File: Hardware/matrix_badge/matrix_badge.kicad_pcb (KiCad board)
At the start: 2 copper layers, 25.4 x 39.4 mm, 35 parts, among them J1 Conn_02x03_Odd_Even, U1 ATTINY85-20SU

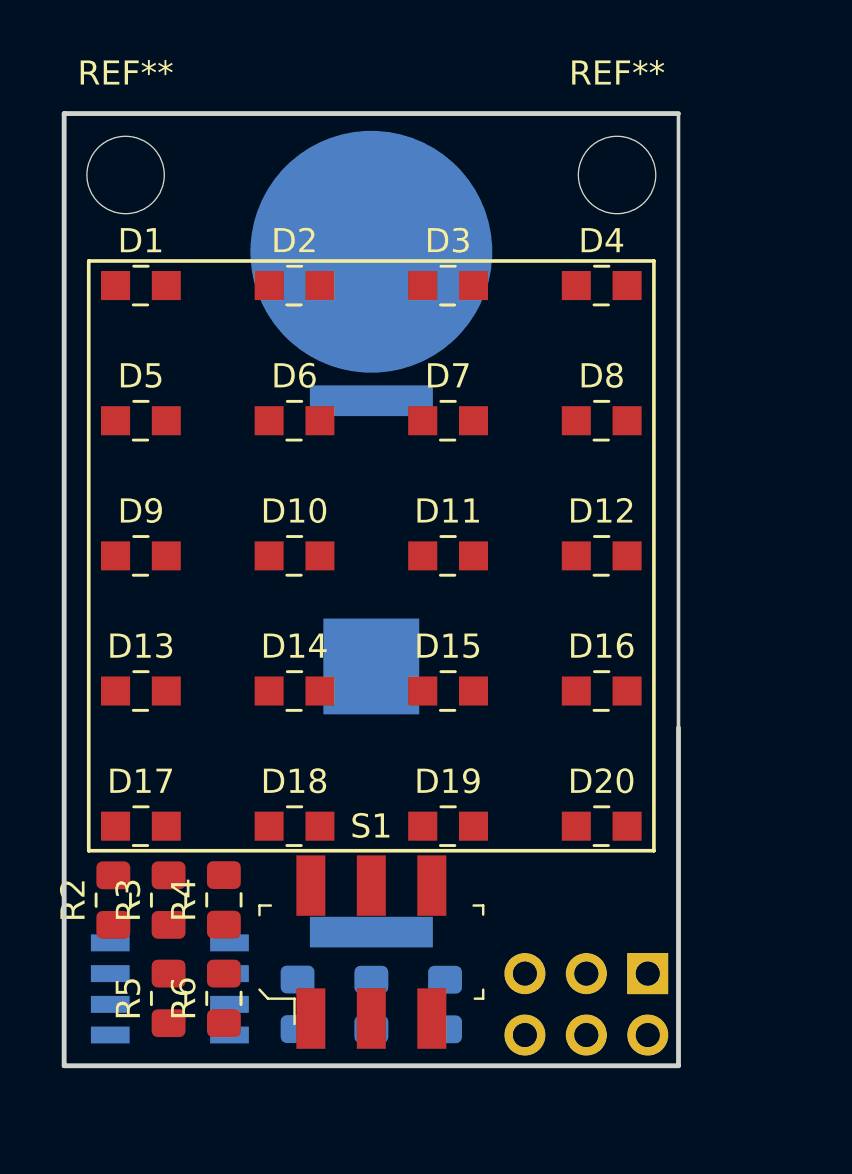
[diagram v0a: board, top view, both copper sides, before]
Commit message: Reconfigured footprint positions
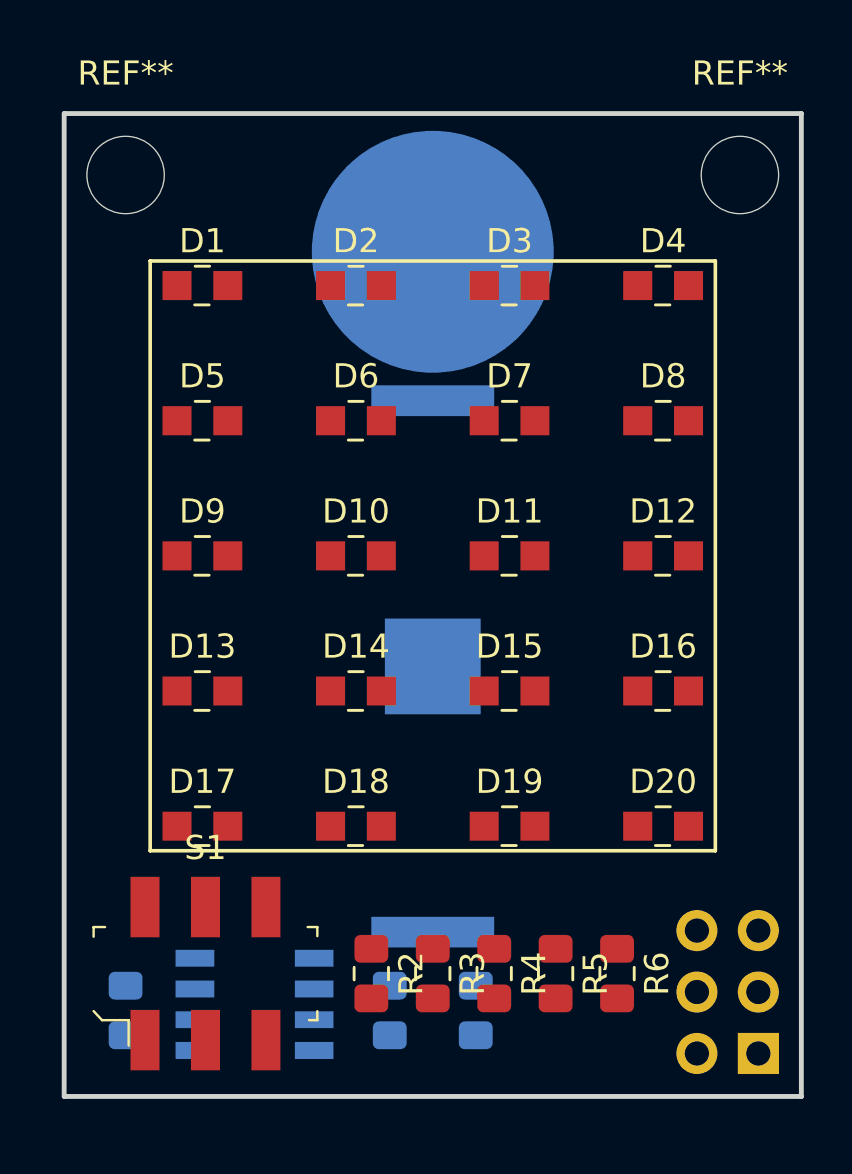
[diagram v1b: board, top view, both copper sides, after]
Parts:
- moved R6 16.3 mm to (149.9, 111.8), turned to 270 degrees
- moved R5 16.0 mm to (147.3, 111.8), turned to 270 degrees
- moved R4 11.6 mm to (144.8, 111.8), turned to 270 degrees
- moved R3 11.3 mm to (142.2, 111.8), turned to 270 degrees
- moved R2 11.1 mm to (139.7, 111.8), turned to 270 degrees
- moved C2 7.12 mm to (129.5, 113.3), turned to 270 degrees
- moved S1 6.92 mm to (132.8, 111.8)
- moved J1 5.64 mm to (155.7, 115.1), turned to 0 degrees
- moved REF** 5.08 mm to (154.9, 78.7)
- moved U1 3.56 mm to (134.9, 113.0)
- moved BT1 2.54 mm to (142.2, 99.1)
- moved REF** 2.54 mm to (142.2, 81.9)
- moved D1 2.54 mm to (132.7, 83.3)
- moved D10 2.54 mm to (139.1, 94.5)
- moved D11 2.54 mm to (145.4, 94.5)
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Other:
- board size 25.4 x 39.4 mm -> 30.5 x 40.6 mm

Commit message: Layout ALMOST done. Missing 1 gnd connection.
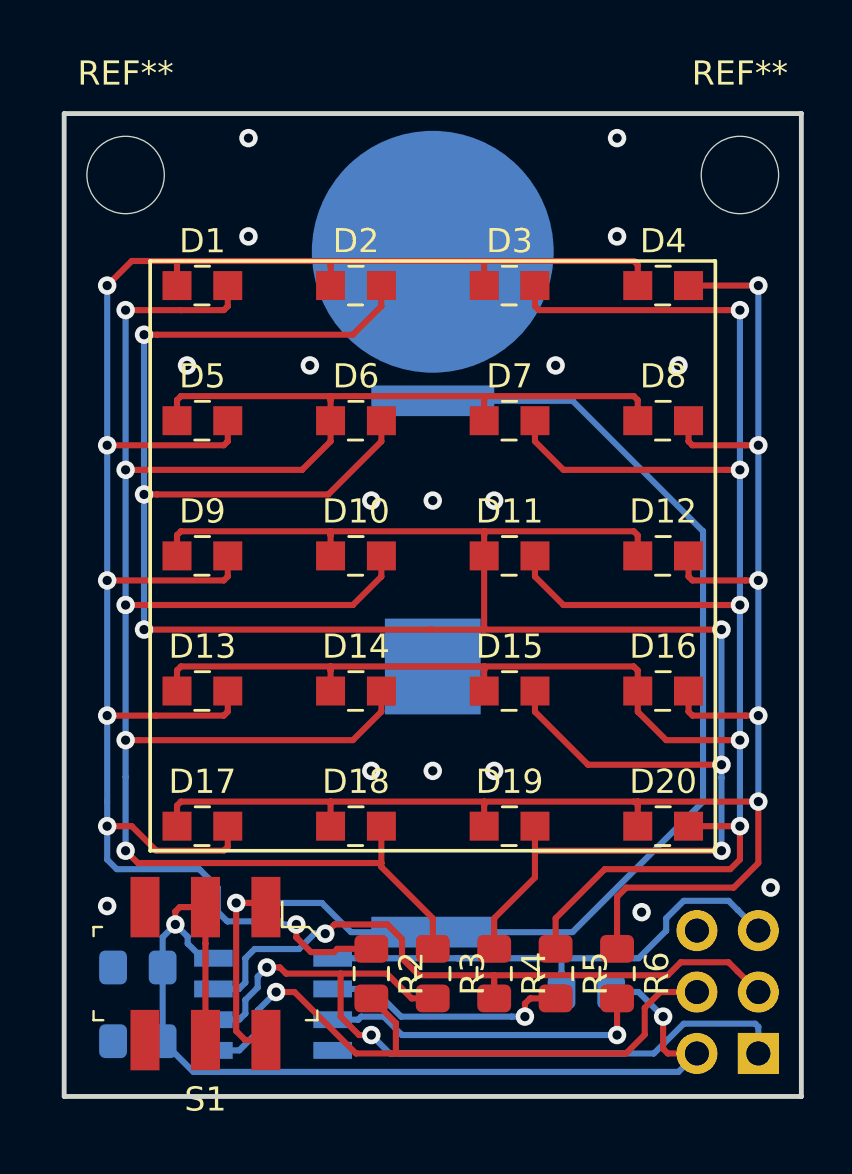
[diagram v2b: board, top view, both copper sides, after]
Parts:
- moved C1 10.5 mm to (130.0, 114.6), turned to 180 degrees
- moved R1 4.64 mm to (148.6, 112.5), turned to 180 degrees
- moved C2 1.85 mm to (130.0, 111.5), turned to 180 degrees
- moved U1 0.76 mm to (135.6, 113.0)
- turned S1 to 180 degrees
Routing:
- net P3: track 0.00 -> 116.9 mm, vias 0 -> 6
- net P2: track 0.00 -> 100.8 mm, vias 0 -> 5
- net P4: track 0.00 -> 92.3 mm, vias 0 -> 5
- net P1: track 0.00 -> 87.6 mm, vias 0 -> 6
- net P5: track 0.00 -> 74.8 mm, vias 0 -> 5
- net Net-(BT1-Pad1): track 0.00 -> 54.7 mm, vias 0 -> 1
- net VDD: track 0.00 -> 43.1 mm, vias 0 -> 2
- net MISO: track 0.00 -> 33.2 mm, vias 0 -> 2
- net SCK: track 0.00 -> 27.2 mm, vias 0 -> 1
- net MOSI: track 0.00 -> 27.0 mm, vias 0 -> 1
- net ~RST: track 0.00 -> 20.8 mm
- net Net-(R6-Pad2): track 0.00 -> 13.6 mm, vias 0 -> 1
- net Net-(R5-Pad2): track 0.00 -> 10.3 mm, vias 0 -> 1
- net GND: vias 0 -> 17
- added copper zone on B.Cu, net GND
- added copper zone on F.Cu, net GND
